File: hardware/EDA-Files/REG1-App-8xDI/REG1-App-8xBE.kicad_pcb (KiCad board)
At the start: 2 copper layers, 83 x 32.8 mm, 4 parts, among them J1 REG1_App_Connector, J10 Conn_01x08, J20 Conn_01x08

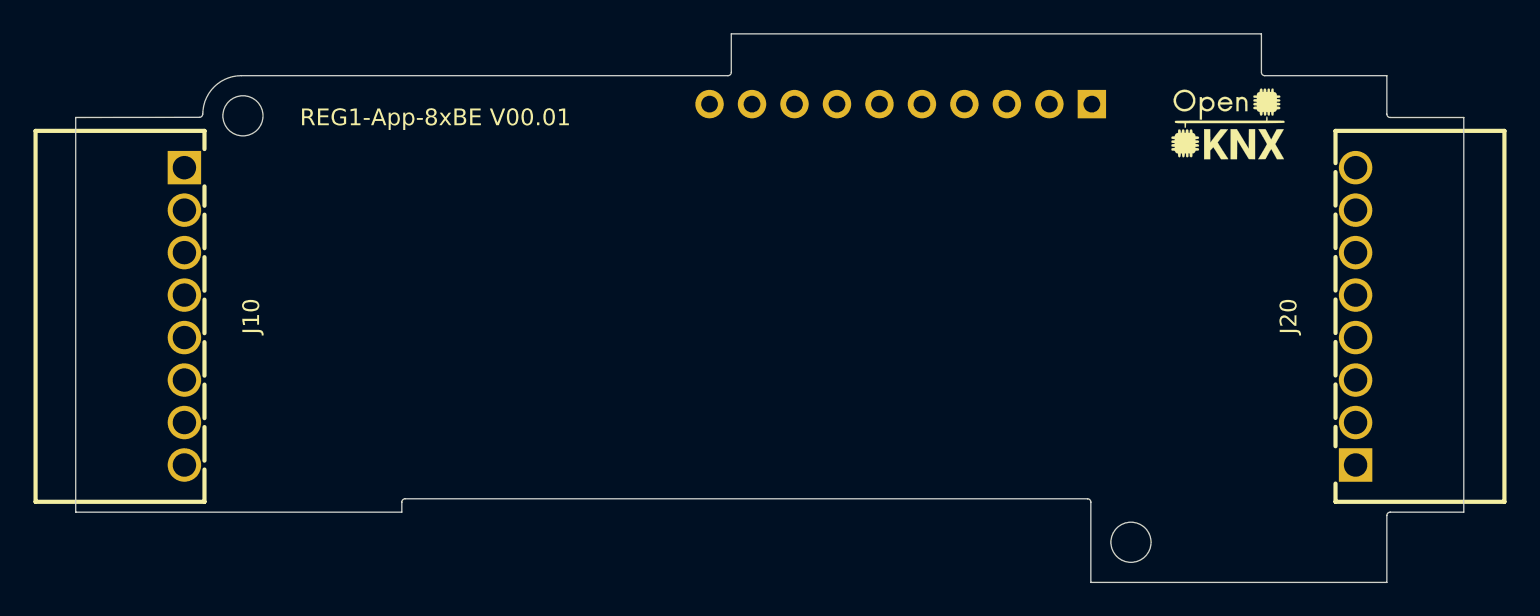
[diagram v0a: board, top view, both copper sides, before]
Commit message: wip 8xBE
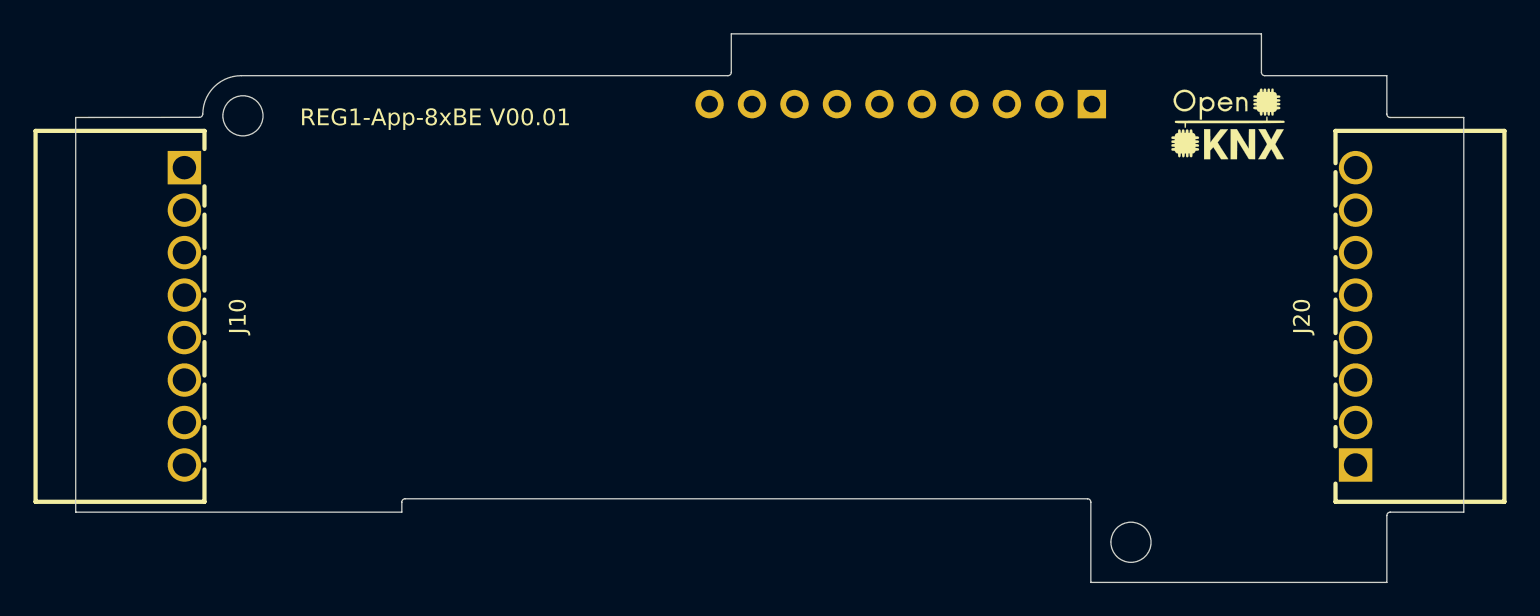
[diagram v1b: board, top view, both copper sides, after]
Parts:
- J10, J20: footprint EasyEDALib:C2927509_CONN-TH_8P-P2.54_DIBO_DB2ERC-2.54-8P-GN -> EasyEDALib:CONN-TH_8P-P2.54_DIBO_DB2ERC-2.54-8P-GN
